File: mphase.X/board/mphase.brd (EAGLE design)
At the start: 120.6 x 82.2 mm, 36 parts, among them IC1 MAX232, IC2 PIC18F4455_40, X1 332-10, X2 332-10

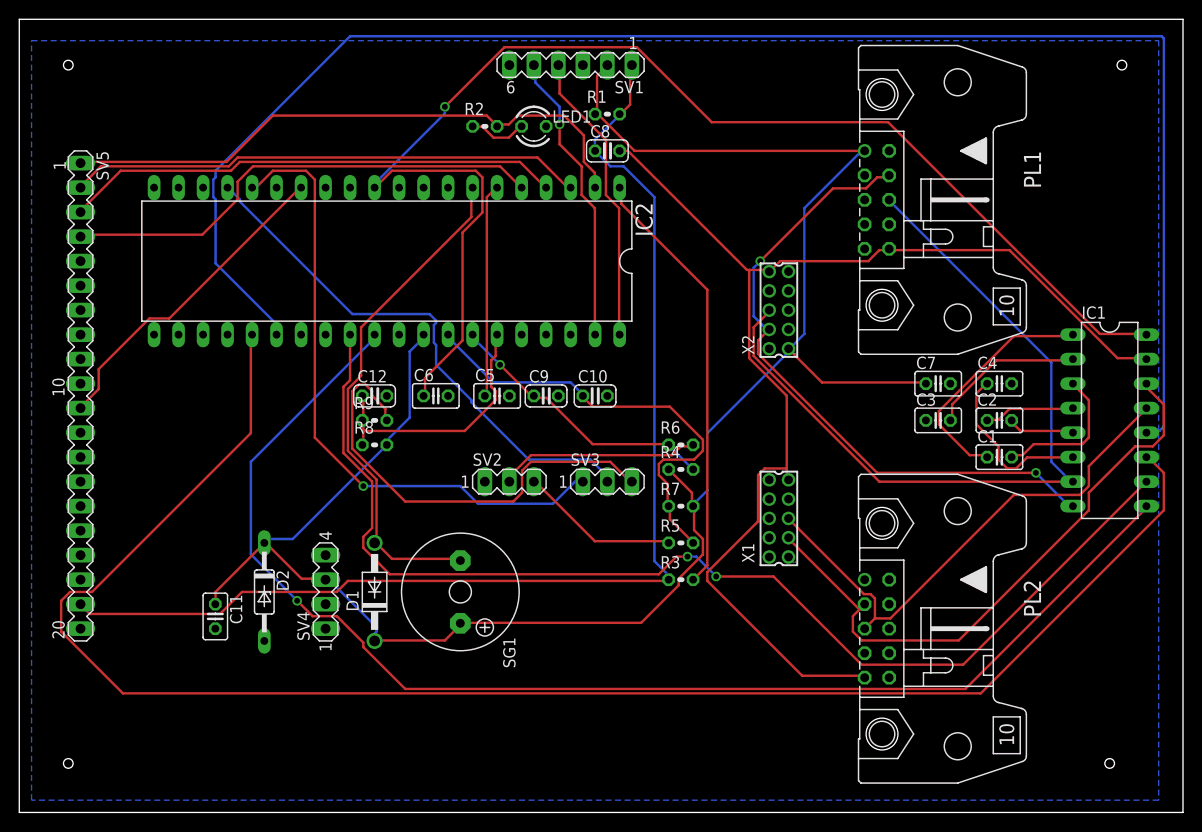
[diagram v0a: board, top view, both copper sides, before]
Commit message: up
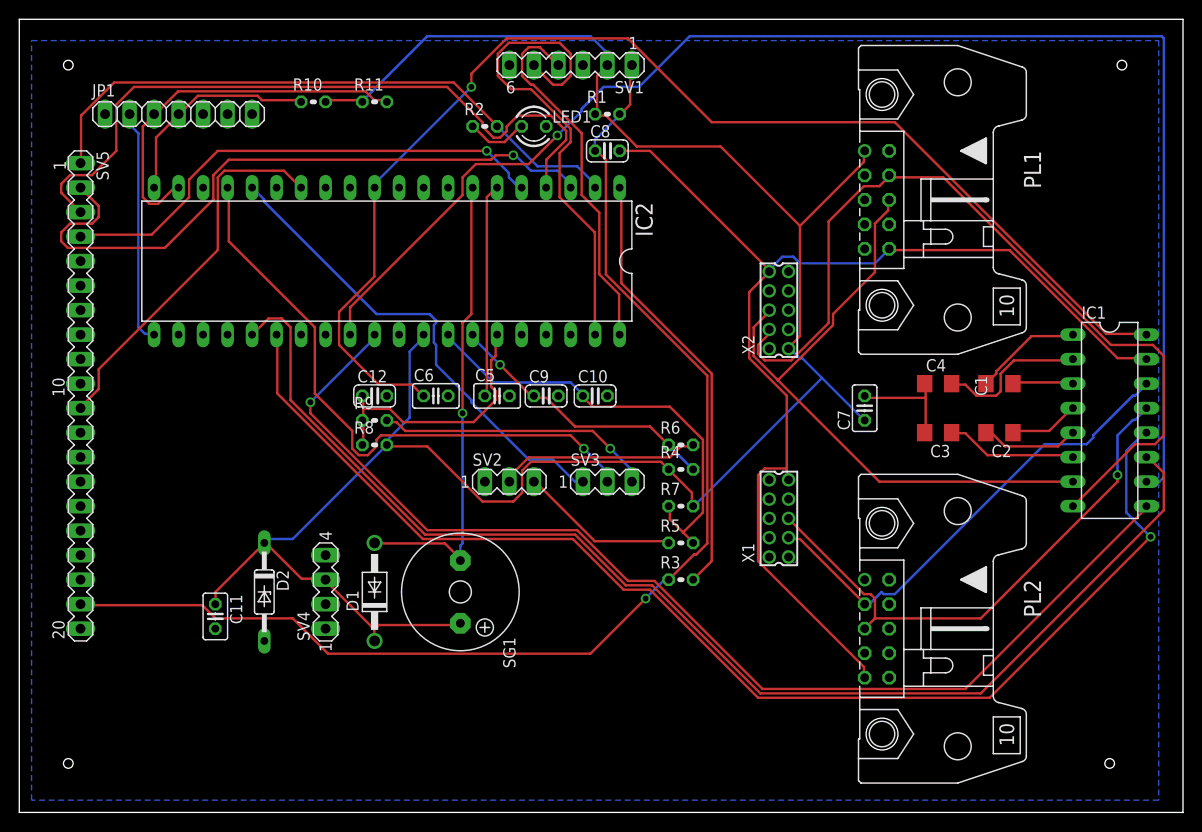
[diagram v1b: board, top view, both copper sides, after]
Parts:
- added JP1: (no value), pinhead:1X07
- added R10, R11: 2.2k, resistor:0204V
- C1, C2, C3, C4: device resistor:C025-025X050 -> rcl:C1206
- moved C7 8.03 mm to (87.6, 41.9), turned to 90 degrees
- moved C1 7.62 mm to (101.6, 44.5)
- moved C4 6.35 mm to (95.2, 44.5)
- moved C2 1.27 mm to (101.6, 39.4), turned to 180 degrees
- moved C3 1.27 mm to (95.2, 39.4), turned to 180 degrees
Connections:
- new net N$37: IC2.21, JP1.2
- new net RD0: IC2.19, JP1.3, R11.2
- new net RD1: IC2.20, JP1.4, R10.1
- net N$5: now also C4.2; no longer C3.2
- net N$6: now also C3.1; no longer C4.1
- net VDD: now also R10.2, R11.1
- net VSS: now also C3.2, C4.1, JP1.6, JP1.7; no longer C3.1, C4.2
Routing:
- net N$11: track 171.5 -> 129.9 mm
- net RD0: track 0.00 -> 39.3 mm
- net N$12: track 166.3 -> 129.7 mm, vias 0 -> 1
- net N$10: track 119.6 -> 147.6 mm, vias 2 -> 1
- net VDD: track 199.4 -> 223.9 mm
- net N$37: track 0.00 -> 24.4 mm
- net N$26: track 51.6 -> 74.1 mm
- net RD1: track 0.00 -> 22.4 mm
- net N$32: track 30.6 -> 51.3 mm, vias 1 -> 0
- net N$17: track 67.6 -> 88.0 mm, vias 2 -> 0
- net N$31: track 47.4 -> 28.9 mm, vias 0 -> 1
- net N$13: track 134.9 -> 117.3 mm
- net N$23: track 53.5 -> 69.4 mm, vias 0 -> 1
- net N$33: track 65.9 -> 50.0 mm, vias 1 -> 0
- net N$16: track 81.1 -> 67.4 mm
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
